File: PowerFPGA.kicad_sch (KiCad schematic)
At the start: 40 parts, among them Q4 Q_NPN_BEC, Q5 Q_PMOS_GDS, U12 EA3059

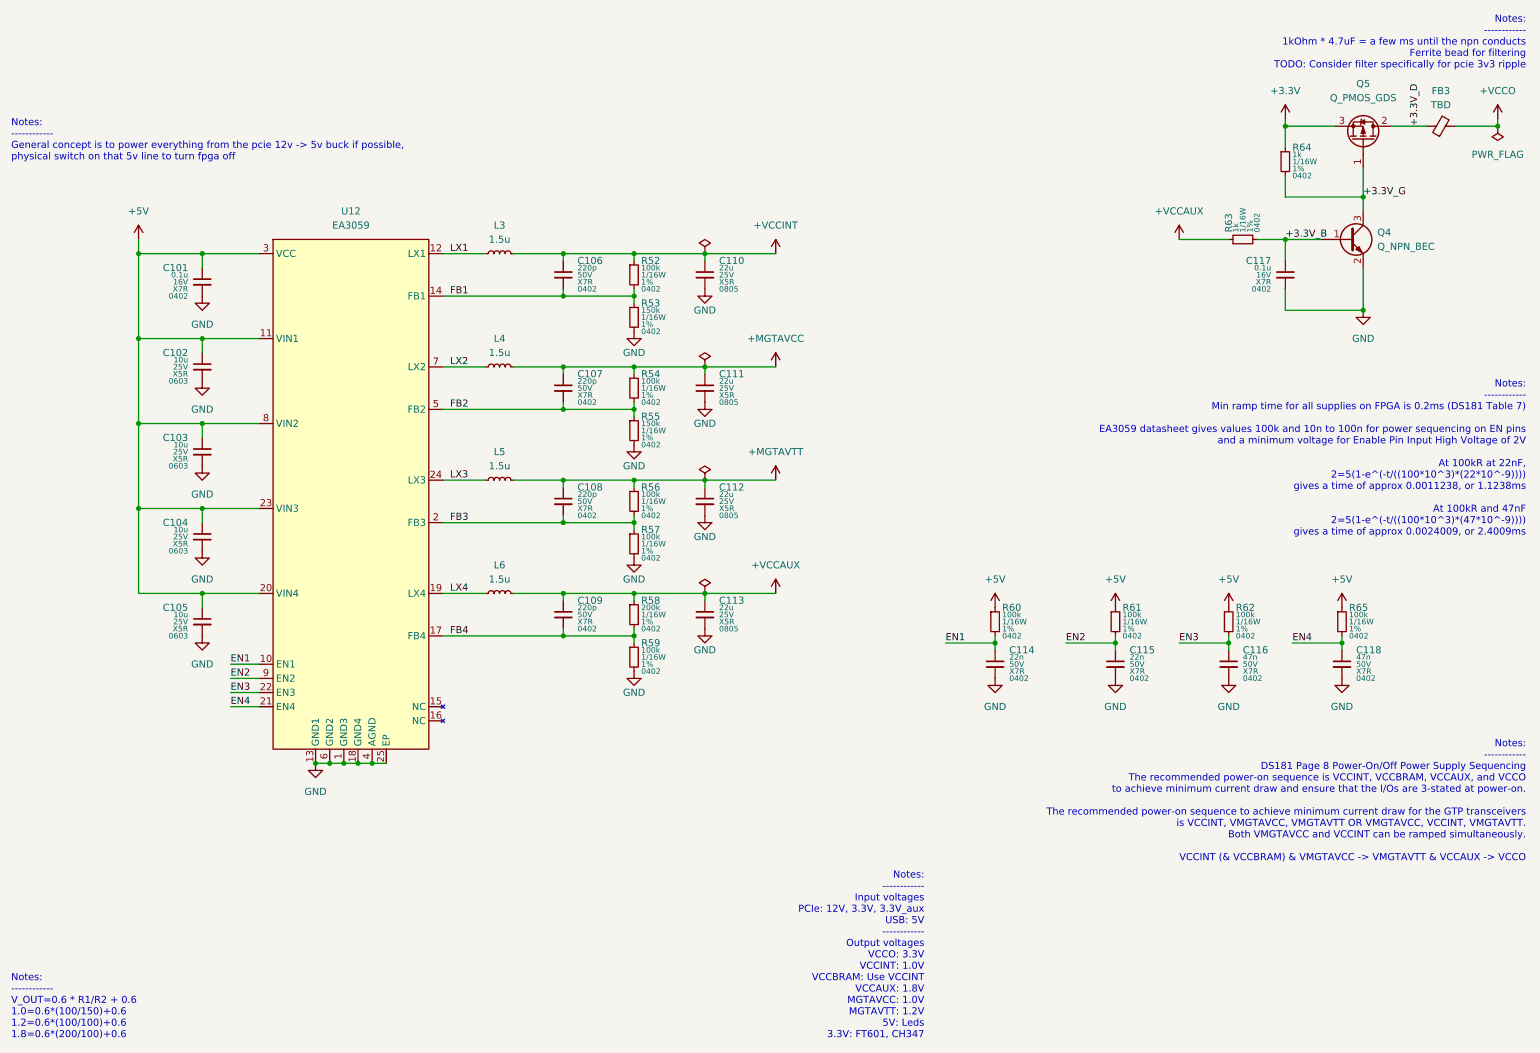
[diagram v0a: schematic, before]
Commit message: Second pass
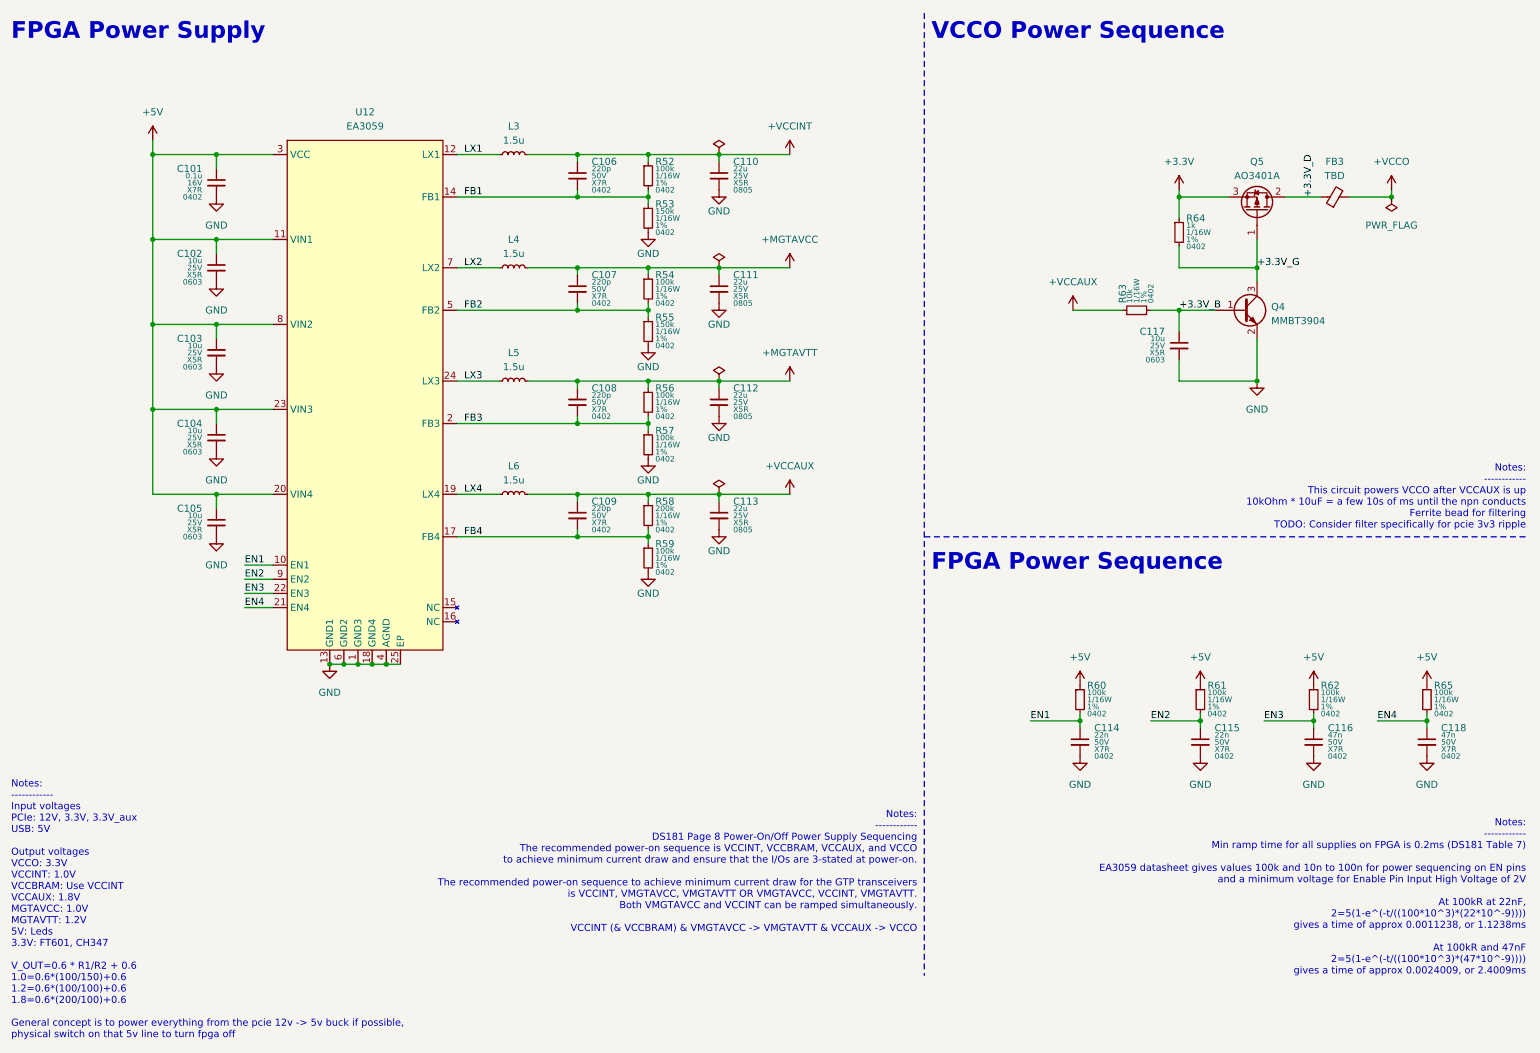
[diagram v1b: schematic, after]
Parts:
- removed Q4: Q_NPN_BEC, Package_TO_SOT_SMD:SOT-23, symbol Device:Q_NPN_BEC
- added Q4: MMBT3904, Package_TO_SOT_SMD:SOT-23, symbol Transistor_BJT:MMBT3904
- C117: value 0.1u -> 10u; footprint Capacitor_SMD:C_0402_1005Metric -> Capacitor_SMD:C_0603_1608Metric; Class X7R -> X5R; Rating 16V -> 25V; Size 0402 -> 0603
- Q5: value Q_PMOS_GDS -> AO3401A
- R63: value 1k -> 10k
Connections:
- net +3.3V_B: now also Q4.1 (B)
- net +3.3V_G: now also Q4.3 (C)
- net GND: now also Q4.2 (E)
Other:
- note added: "FPGA Power Sequence"
- note added: "FPGA Power Supply"
- note added: "Notes: ------------ Input voltages PCIe: 12V, 3.3V, 3.3V_aux USB: 5V Output voltages VCCO: 3.3V VCCINT: 1.0V VCCBRAM: Use VCCINT VCCAUX: 1.8V MGTAVCC: 1.0V MGTAVTT: 1.2V 5V: Leds 3.3V: FT601, CH347 V_OUT=0.6 * R1/R2 + 0.6 1.0=0.6*(100/150)+0.6 1.2=0.6*(100/100)+0.6 1.8=0.6*(200/100)+0.6 General concept is to power everything from the pcie 12v -> 5v buck if possible, physical switch on that 5v lin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"
- note added: "Notes: ------------ This circuit powers VCCO after VCCAUX is up 10kOhm * 10uF = a few 10s of ms until the npn conducts Ferrite bead for filtering TODO: Consider filter specifically for pcie 3v3 ripple"
- note added: "VCCO Power Sequence"
- note removed: "Notes: ------------ 1kOhm * 4.7uF = a few ms until the npn conducts Ferrite bead for filtering TODO: Consider filter specifically for pcie 3v3 ripple"
- note removed: "Notes: ------------ General concept is to power everything from the pcie 12v -> 5v buck if possible, physical switch on that 5v line to turn fpga off"
- note removed: "Notes: ------------ Input voltages PCIe: 12V, 3.3V, 3.3V_aux USB: 5V ------------ Output voltages VCCO: 3.3V VCCINT: 1.0V VCCBRAM: Use VCCINT VCCAUX: 1.8V MGTAVCC: 1.0V MGTAVTT: 1.2V 5V: Leds 3.3V: FT601, CH347"
- note removed: "Notes: ------------ V_OUT=0.6 * R1/R2 + 0.6 1.0=0.6*(100/150)+0.6 1.2=0.6*(100/100)+0.6 1.8=0.6*(200/100)+0.6"
- moved on the sheet: C101, C102, C103, C104, C105, C106, C107, C108, C109, C110, C111, C112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

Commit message: Third pass
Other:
- company: (none) -> github.com/eggsampler
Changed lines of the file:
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@@
     (date "2024-01-01")
     (rev "1")
+    (company "github.com/eggsampler")
   )
   (junction (at 49.53 53.34) (diameter 0) (color 0 0 0 0)
